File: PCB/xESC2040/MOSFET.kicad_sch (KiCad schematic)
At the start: 6 parts, among them J10 Conn_02x02_Counter_Clockwise, Q5 BSC026N08NS5, Q6 BSC026N08NS5

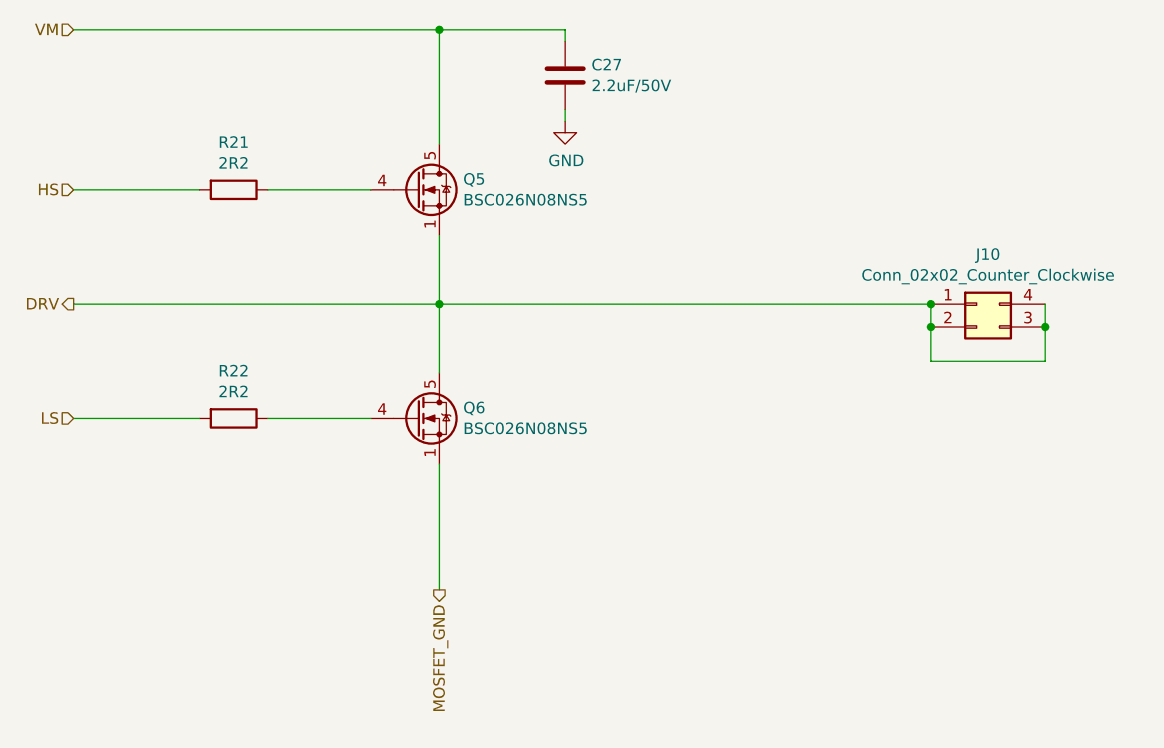
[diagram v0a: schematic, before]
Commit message: wip
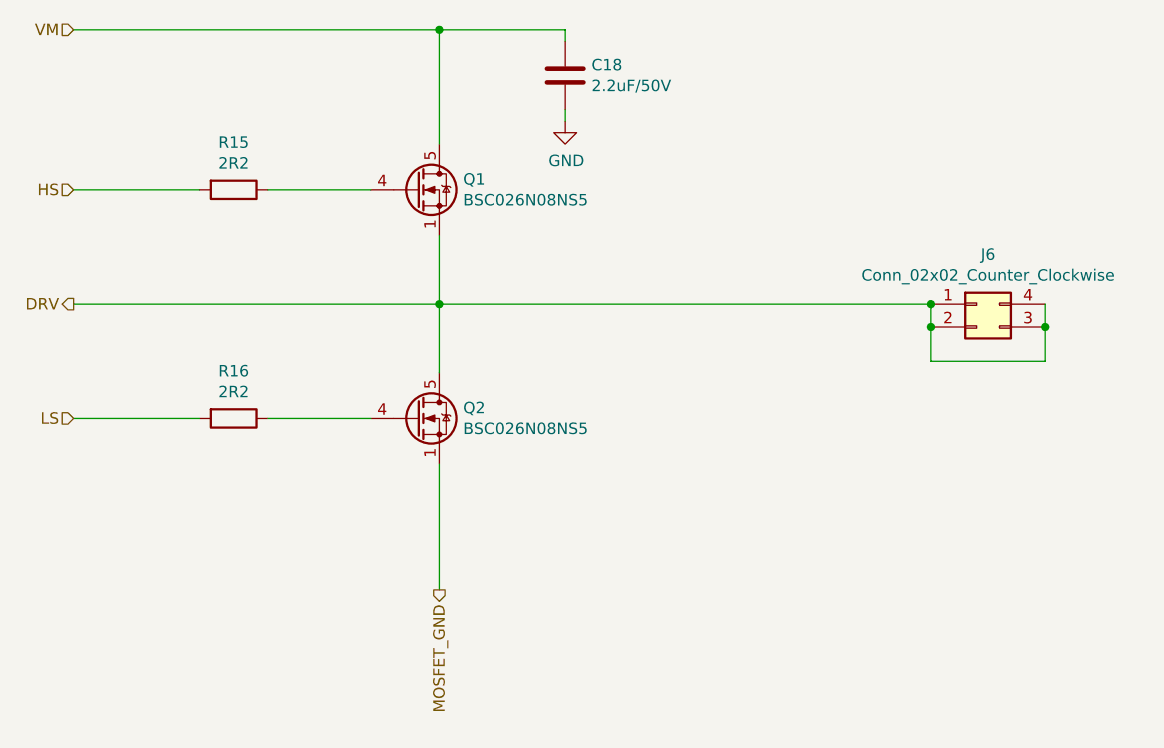
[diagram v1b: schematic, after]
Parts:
- renumbered C27 to C18, J10 to J6, Q5 to Q1, Q6 to Q2, R21 to R15, R22 to R16
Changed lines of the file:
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@@
     (effects (font (size 1.27 1.27)) (justify right))
   )
-  (symbol (lib_id "Transistor_FET:BSC026N08NS5") (at 173.99 71.12 0)
+  (symbol (lib_id "Transistor_FET:BSC026N08NS5") (at 173.99 71.12 0) (unit 1)
     (in_bom yes) (on_board yes)
-    (property "Reference" "Q5" (id 0) (at 179.1716 69.9516 0)
+    (property "Reference" "Q1" (id 0) (at 179.1716 69.9516 0)
       (effects (font (size 1.27 1.27)) (justify left))
     )
@@
     (pin "5")
   )
-  (symbol (lib_id "Transistor_FET:BSC026N08NS5") (at 173.99 96.52 0)
+  (symbol (lib_id "Transistor_FET:BSC026N08NS5") (at 173.99 96.52 0) (unit 1)
     (in_bom yes) (on_board yes)
-    (property "Reference" "Q6" (id 0) (at 179.1716 95.3516 0)
+    (property "Reference" "Q2" (id 0) (at 179.1716 95.3516 0)
       (effects (font (size 1.27 1.27)) (justify left))
     )
@@
     (pin "5")
   )
-  (symbol (lib_id "Device:R") (at 153.67 71.12 270)
+  (symbol (lib_id "Device:R") (at 153.67 71.12 270) (unit 1)
     (in_bom yes) (on_board yes)
-    (property "Reference" "R21" (id 0) (at 153.67 65.8622 90))
+    (property "Reference" "R15" (id 0) (at 153.67 65.8622 90))
     (property "Value" "2R2" (id 1) (at 153.67 68.1736 90))
     (property "Footprint" "Resistor_SMD:R_0603_1608Metric" (id 2) (at 153.67 69.342 90)
@@
     (pin "2")
   )
-  (symbol (lib_id "Device:R") (at 153.67 96.52 270)
+  (symbol (lib_id "Device:R") (at 153.67 96.52 270) (unit 1)
     (in_bom yes) (on_board yes)
-    (property "Reference" "R22" (id 0) (at 153.67 91.2622 90))
+    (property "Reference" "R16" (id 0) (at 153.67 91.2622 90))
     (property "Value" "2R2" (id 1) (at 153.67 93.5736 90))
     (property "Footprint" "Resistor_SMD:R_0603_1608Metric" (id 2) (at 153.67 94.742 90)
@@
     (pin "2")
   )
-  (symbol (lib_id "Device:C") (at 190.5 58.42 0)
+  (symbol (lib_id "Device:C") (at 190.5 58.42 0) (unit 1)
     (in_bom yes) (on_board yes)
-    (property "Reference" "C27" (id 0) (at 193.421 57.2516 0)
+    (property "Reference" "C18" (id 0) (at 193.421 57.2516 0)
       (effects (font (size 1.27 1.27)) (justify left))
     )
@@
     (pin "2")
   )
-  (symbol (lib_id "power:GND") (at 190.5 63.5 0)
+  (symbol (lib_id "power:GND") (at 190.5 63.5 0) (unit 1)
     (in_bom yes) (on_board yes)
-    (property "Reference" "#PWR037" (id 0) (at 190.5 69.85 0)
+    (property "Reference" "#PWR022" (id 0) (at 190.5 69.85 0)
       (effects (font (size 1.27 1.27)) hide)
     )
@@
     (pin "1")
   )
-  (symbol (lib_id "Connector_Generic:Conn_02x02_Counter_Clockwise") (at 236.22 83.82 0)
+  (symbol (lib_id "Connector_Generic:Conn_02x02_Counter_Clockwise") (at 236.22 83.82 0) (unit 1)
     (in_bom yes) (on_board yes)
-    (property "Reference" "J10" (id 0) (at 237.49 78.3082 0))
+    (property "Reference" "J6" (id 0) (at 237.49 78.3082 0))
     (property "Value" "Conn_02x02_Counter_Clockwise" (id 1) (at 237.49 80.6196 0))
     (property "Footprint" "Connector_PinHeader_2.54mm:PinHeader_2x02_P2.54mm_Vertical" (id 2) (at 236.22 83.82 0)
